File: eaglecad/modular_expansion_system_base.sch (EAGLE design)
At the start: 40 parts, among them IC1 74LS244N, IC10 74LS30N, IC2 74LS244N, IC3 74LS244N, IC4 SRAM, IC5 74LS30N, IC6 LM2596T-5.0, IC8 74LS00N, IC9 7805T, J1-INTERRUPTS INTERRUPTS, J1_ADDRESS_CON j1, J2-WAITS WAITS, J2_DATA_AND_POWER_CON j2, SW1 100SP3T1B1M6QE

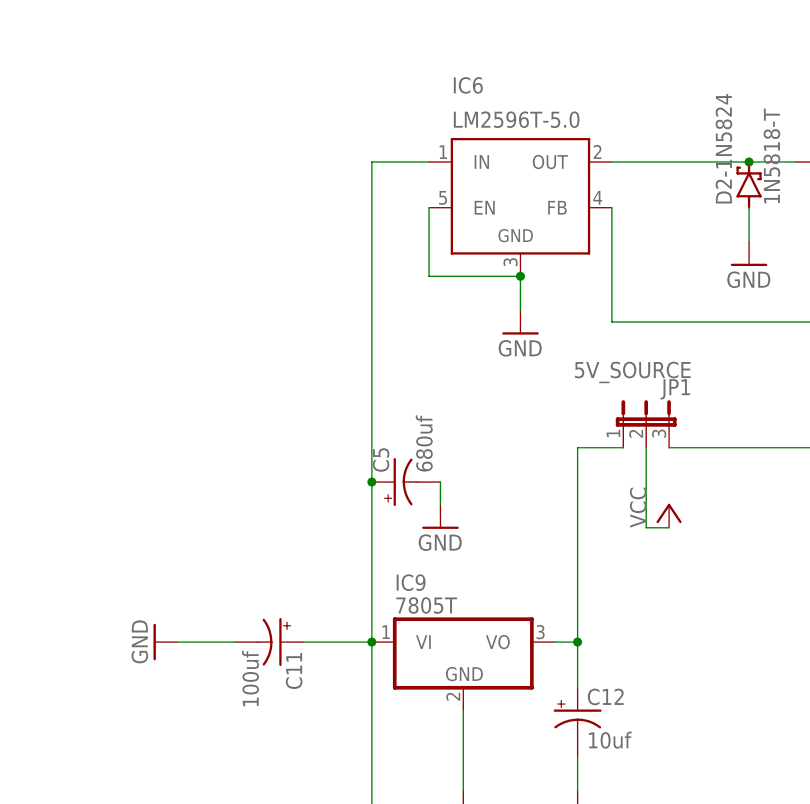
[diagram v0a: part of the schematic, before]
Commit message: added bill of materials
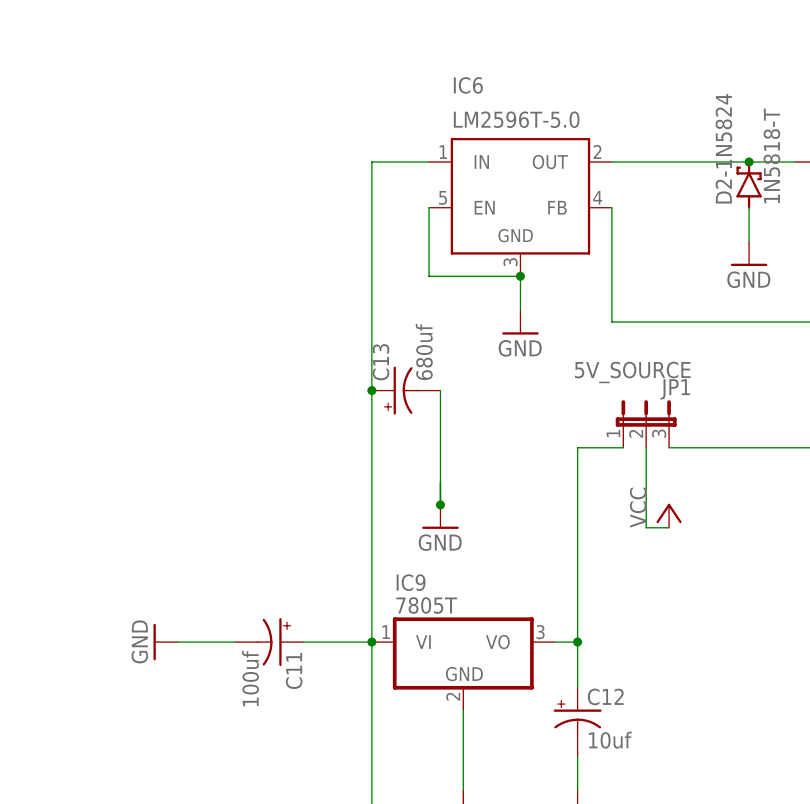
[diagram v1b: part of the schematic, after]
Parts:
- removed C5: 680uf, rcl:CPOL-USE2.5-5
- added C13: 680uf, rcl:CPOL-USE3.5-8
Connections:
- net 9V-POST-SW: now also C13.+; no longer C5.+
- net GND: now also C13.-; no longer C5.-
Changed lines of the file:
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@@
 <part name="IC6" library="linear" library_urn="urn:adsk.eagle:library:262" deviceset="LM2596T" device="H" package3d_urn="urn:adsk.eagle:package:16443/1" value="LM2596T-5.0"/>
 <part name="GND10" library="supply1" library_urn="urn:adsk.eagle:library:371" deviceset="GND" device=""/>
-<part name="C5" library="rcl" library_urn="urn:adsk.eagle:library:334" deviceset="CPOL-US" device="E2.5-5" package3d_urn="urn:adsk.eagle:package:23344/1" value="680uf"/>
 <part name="GND11" library="supply1" library_urn="urn:adsk.eagle:library:371" deviceset="GND" device=""/>
 <part name="D2-1N5824" library="diode" library_urn="urn:adsk.eagle:library:210" deviceset="1N581*" device="" package3d_urn="urn:adsk.eagle:package:43421/1" technology="8-T"/>
@@
 <part name="JP1" library="jumper" library_urn="urn:adsk.eagle:library:252" deviceset="JP2E" device="" package3d_urn="urn:adsk.eagle:package:15452/1" value="5V_SOURCE"/>
 <part name="P+7" library="supply1" library_urn="urn:adsk.eagle:library:371" deviceset="VCC" device=""/>
+<part name="C13" library="rcl" library_urn="urn:adsk.eagle:library:334" deviceset="CPOL-US" device="E3.5-8" package3d_urn="urn:adsk.eagle:package:23360/2" value="680uf"/>
 </parts>
 <sheets>
@@
 <attribute name="VALUE" x="59.69" y="92.71" size="1.778" layer="96"/>
 </instance>
-<instance part="C5" gate="G$1" x="48.26" y="78.74" smashed="yes" rot="R90">
-<attribute name="NAME" x="47.625" y="79.756" size="1.778" layer="95" rot="R90"/>
-<attribute name="VALUE" x="52.451" y="79.756" size="1.778" layer="96" rot="R90"/>
-</instance>
 <instance part="GND11" gate="1" x="53.34" y="73.66" smashed="yes">
 <attribute name="VALUE" x="50.8" y="71.12" size="1.778" layer="96"/>
@@
 <instance part="P+7" gate="VCC" x="78.74" y="76.2" smashed="yes">
 <attribute name="VALUE" x="76.2" y="73.66" size="1.778" layer="96" rot="R90"/>
+</instance>
+<instance part="C13" gate="G$1" x="48.26" y="88.9" smashed="yes" rot="R90">
+<attribute name="NAME" x="47.625" y="89.916" size="1.778" layer="95" rot="R90"/>
+<attribute name="VALUE" x="52.451" y="89.916" size="1.778" layer="96" rot="R90"/>
 </instance>
 </instances>
@@
 </segment>
 <segment>
-<pinref part="C5" gate="G$1" pin="-"/>
 <pinref part="GND11" gate="1" pin="GND"/>
 <wire x1="53.34" y1="78.74" x2="53.34" y2="76.2" width="0.1524" layer="91"/>
+<pinref part="C13" gate="G$1" pin="-"/>
+<wire x1="53.34" y1="88.9" x2="53.34" y2="76.2" width="0.1524" layer="91"/>
+<junction x="53.34" y="76.2"/>
 </segment>
 <segment>
@@
 <pinref part="IC6" gate="NC1" pin="IN"/>
 <wire x1="52.07" y1="114.3" x2="45.72" y2="114.3" width="0.1524" layer="91"/>
-<wire x1="45.72" y1="114.3" x2="45.72" y2="78.74" width="0.1524" layer="91"/>
-<pinref part="C5" gate="G$1" pin="+"/>
-<wire x1="45.72" y1="78.74" x2="45.72" y2="60.96" width="0.1524" layer="91"/>
-<junction x="45.72" y="78.74"/>
-</segment>
-</net>
+<wire x1="45.72" y1="114.3" x2="45.72" y2="88.9" width="0.1524" layer="91"/>
+<wire x1="45.72" y1="88.9" x2="45.72" y2="60.96" width="0.1524" layer="91"/>
+<pinref part="C13" gate="G$1" pin="+"/>
+<junction x="45.72" y="88.9"/>
+</segment>
+</net>
